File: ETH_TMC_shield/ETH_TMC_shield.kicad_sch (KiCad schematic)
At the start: 52 parts, among them J10 Conn_02x06_Odd_Even, J11 Conn_02x06_Odd_Even, J12 Conn_01x02_Pin, J13 Conn_01x03_Pin, J5 USB_B_Micro, J6 JXD2-0Z10NL, U6 STM32H563RGTx, U9 LAN8742A-CZ-TR, Y2 25Mhz

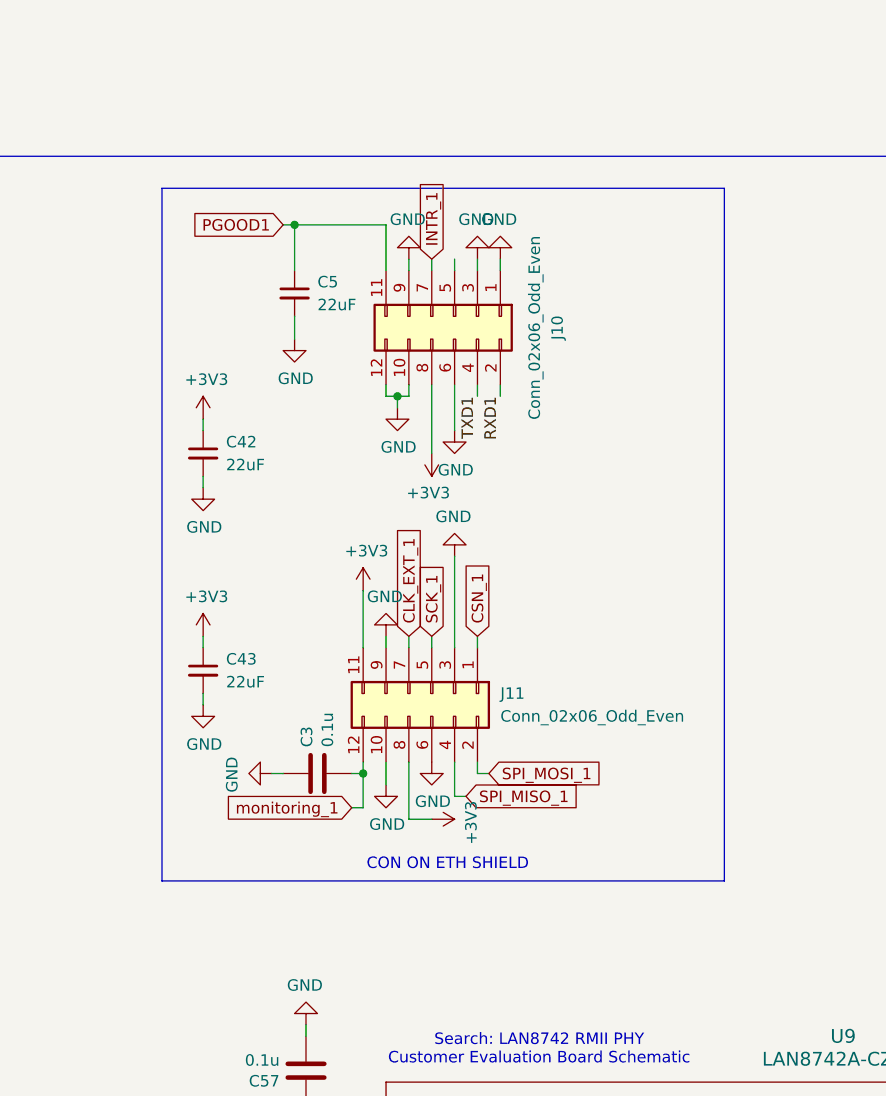
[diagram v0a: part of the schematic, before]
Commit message: finished
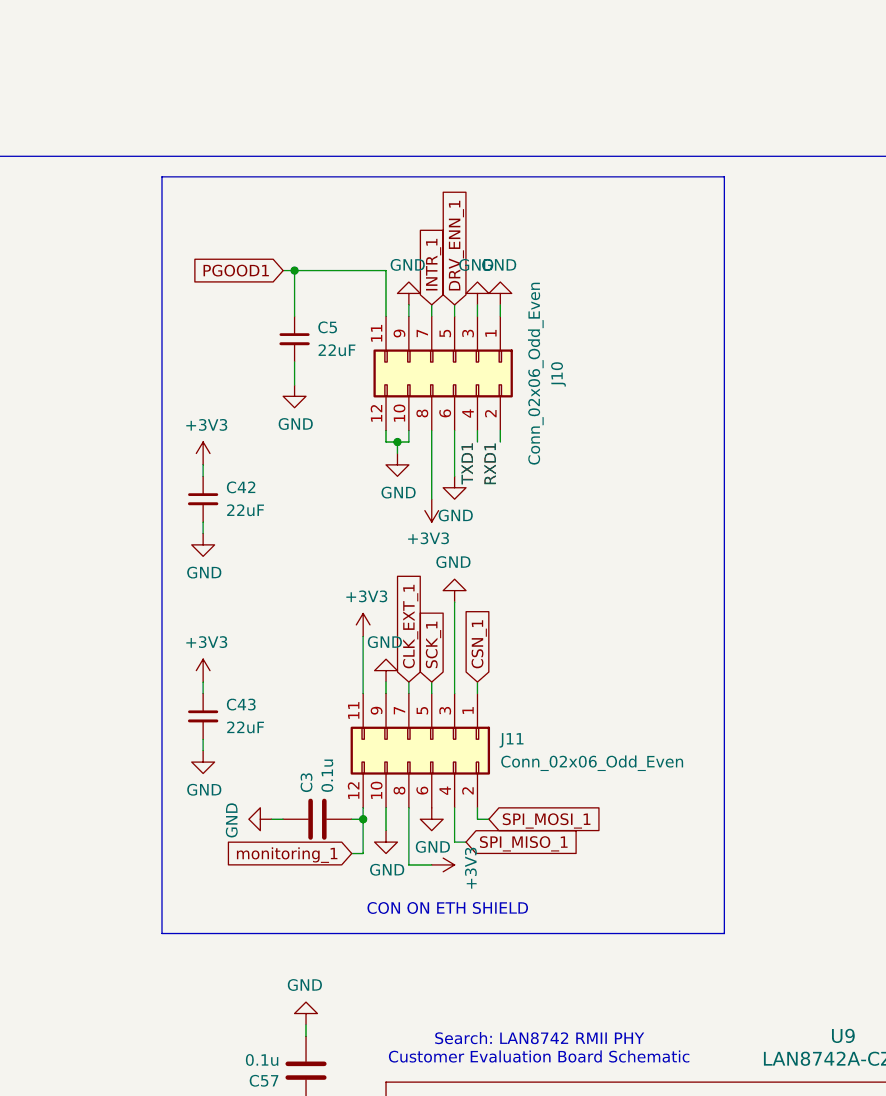
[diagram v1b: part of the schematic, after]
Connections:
- net DRV_ENN_1: now also J10.5 (Pin_5)
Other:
- moved on the sheet: C3, C42, C43, C5, J10, J11
